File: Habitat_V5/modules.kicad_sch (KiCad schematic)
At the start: 34 parts, among them U11 ADS1115IDGS

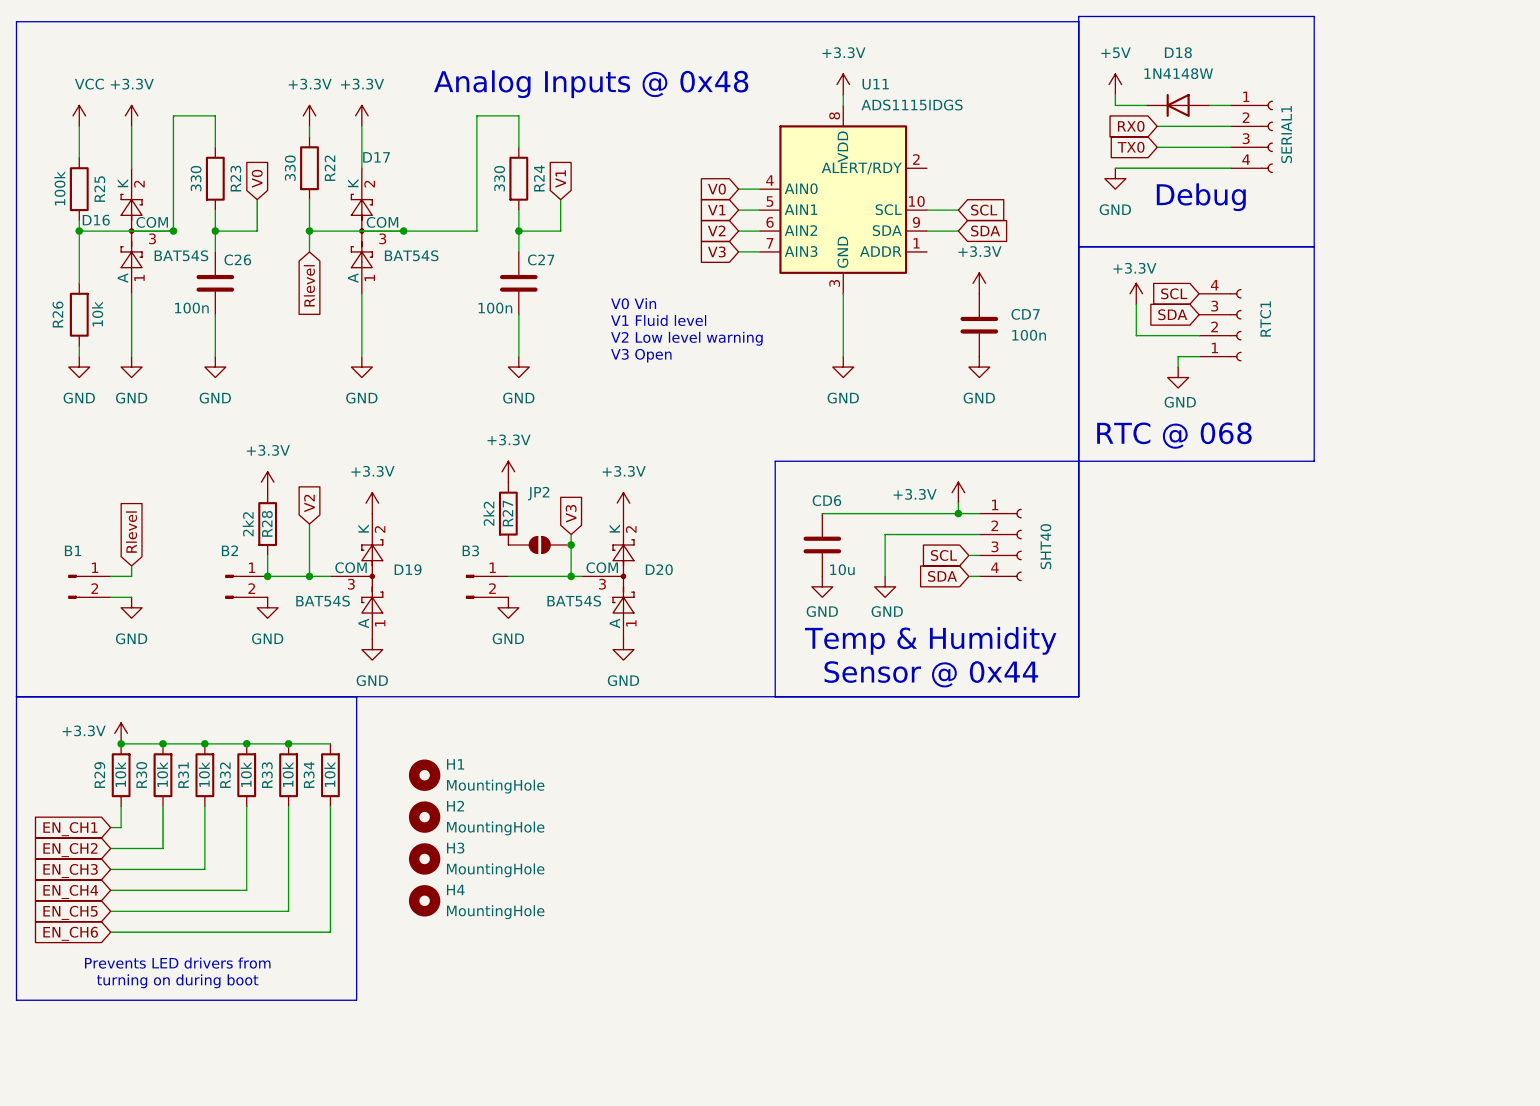
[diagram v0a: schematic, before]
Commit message: Updated PCB and Schematic
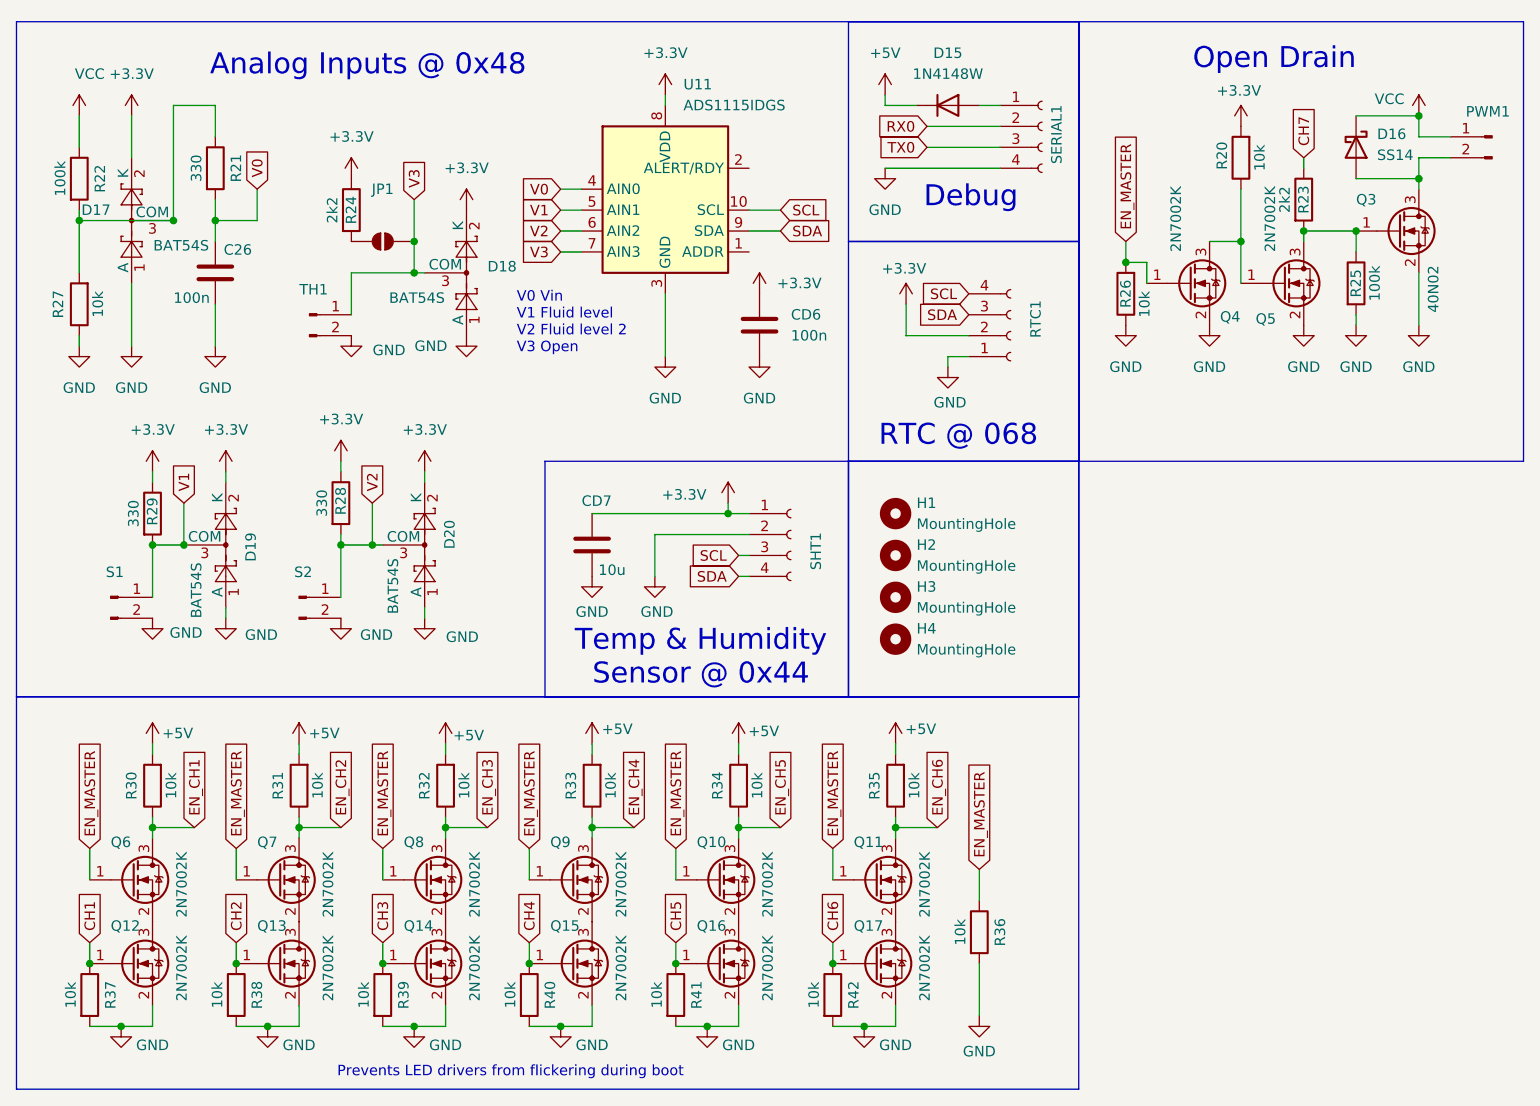
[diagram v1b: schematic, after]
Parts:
- removed C27: 100n, Capacitor_SMD:C_0805_2012Metric, symbol Device:C
- removed R24: 330, Resistor_SMD:R_0805_2012Metric, symbol Device:R
- removed R29: 10k, Resistor_SMD:R_0805_2012Metric, symbol Device:R
- added D16: SS14, Diode_SMD:D_SMA, symbol Diode:SS14
- added PWM1: Conn_01x02_Pin, Connector_Phoenix_MSTB:PhoenixContact_MSTBA_2,5_2-G-5,08_1x02_P5.08mm_Horizontal, symbol Connector:Conn_01x02_Pin
- added Q10, Q11, Q12, Q13, Q14, Q15, Q16, Q17, Q4, Q5, Q6, Q7, Q8, Q9: 2N7002K, Package_TO_SOT_SMD:SOT-23, symbol Transistor_FET:2N7002K
- added Q3: 40N02, Package_TO_SOT_SMD:TO-252-2, symbol Transistor_FET:2N7002K
- added R20, R26, R35, R36, R37, R38, R39, R40, R41, R42: 10k, Resistor_SMD:R_0805_2012Metric, symbol Device:R
- added R23: 2k2, Resistor_SMD:R_0805_2012Metric, symbol Device:R
- added R25: 100k, Resistor_SMD:R_0805_2012Metric, symbol Device:R
- R28: value 2k2 -> 330; LCSC C17520 -> C17630
- S1: renamed from B1; footprint Connector_Molex:Molex_KK-254_AE-6410-02A_1x02_P2.54mm_Vertical -> Connector_Phoenix_MSTB:PhoenixContact_MSTBA_2,5_2-G-5,08_1x02_P5.08mm_Horizontal
- S2: renamed from B2; footprint Connector_Molex:Molex_KK-254_AE-6410-02A_1x02_P2.54mm_Vertical -> Connector_Phoenix_MSTB:PhoenixContact_MSTBA_2,5_2-G-5,08_1x02_P5.08mm_Horizontal
- TH1: renamed from B3; footprint Connector_Molex:Molex_KK-254_AE-6410-02A_1x02_P2.54mm_Vertical -> Connector_Phoenix_MSTB:PhoenixContact_MSTBA_2,5_2-G-5,08_1x02_P5.08mm_Horizontal
- renumbered CD7 to CD6, CD6 to CD7, D18 to D15, D16 to D17, D20 to D18, D17 to D19, D19 to D20, JP2 to JP1, R23 to R21, R25 to R22, R27 to R24, R26 to R27, R22 to R29, SHT40 to SHT1
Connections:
- net Rlevel is gone; now on net V1: D19.3 (COM), R29.2, S1.1 (Pin_1)
- net +3.3V: now also R20.2; no longer R30.2, R31.2, R32.2, R33.2, R34.2
- net +5V: now also R30.2, R31.2, R32.2, R33.2, R34.2, R35.2
- net EN_CH1: now also R30.1, Q6.3 (D)
- net EN_CH2: now also R31.1, Q7.3 (D); no longer R30.1
- net EN_CH3: now also R32.1, Q8.3 (D); no longer R31.1
- net EN_CH4: now also R33.1, Q9.3 (D); no longer R32.1
- net EN_CH5: now also R34.1, Q10.3 (D); no longer R33.1
- net EN_CH6: now also Q11.3 (D), R35.1; no longer R34.1
- net GND: now also Q12.2 (S), Q13.2 (S), Q14.2 (S), Q15.2 (S), Q16.2 (S), Q17.2 (S), Q3.2 (S), Q4.2 (S), Q5.2 (S), R25.2, R26.1, R36.2, R37.2, R38.2, R39.2, R40.2, R41.2, R42.2
- net VCC: now also D16.1 (K), PWM1.1 (Pin_1)
- new net: Q12.3 (D), Q6.2 (S)
- new net: D16.2 (A), PWM1.2 (Pin_2), Q3.3 (D)
- new net: Q3.1 (G), Q5.3 (D), R23.2, R25.1
- new net: Q13.3 (D), Q7.2 (S)
- new net: Q4.3 (D), Q5.1 (G), R20.1
- new net: Q14.3 (D), Q8.2 (S)
- new net: Q11.2 (S), Q17.3 (D)
- new net: Q15.3 (D), Q9.2 (S)
- new net: Q10.2 (S), Q16.3 (D)
- new net CH1: Q12.1 (G), R37.1
- new net CH2: Q13.1 (G), R38.1
- new net CH3: Q14.1 (G), R39.1
- new net CH4: Q15.1 (G), R40.1
- new net CH5: Q16.1 (G), R41.1
- new net CH6: Q17.1 (G), R42.1
- new net CH7: R23.1
- new net EN_MASTER: Q10.1 (G), Q11.1 (G), Q4.1 (G), Q6.1 (G), Q7.1 (G), Q8.1 (G), Q9.1 (G), R26.2, R36.1
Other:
- note added: "Open Drain"
- note added: "Prevents LED drivers from flickering during boot"
- note added: "V0 Vin V1 Fluid level V2 Fluid level 2 V3 Open"
- note removed: "Prevents LED drivers from turning on during boot"
- note removed: "V0 Vin V1 Fluid level V2 Low level warning V3 Open"
- moved on the sheet: C26, CD6, CD7, D15, D17, D18, D19, D20, H1, H2, H3, H4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
